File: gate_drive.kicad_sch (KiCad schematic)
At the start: 110 parts, among them J19 Conn_01x03, J20 Conn_01x03, U1 EG2131, U14 CC6920B, U2 EG2131, U20 CC6920B, U22 CC6920B, U3 CC6920B, U4 EG2131, U5 EG2131, U7 EG2131, U8 EG2131

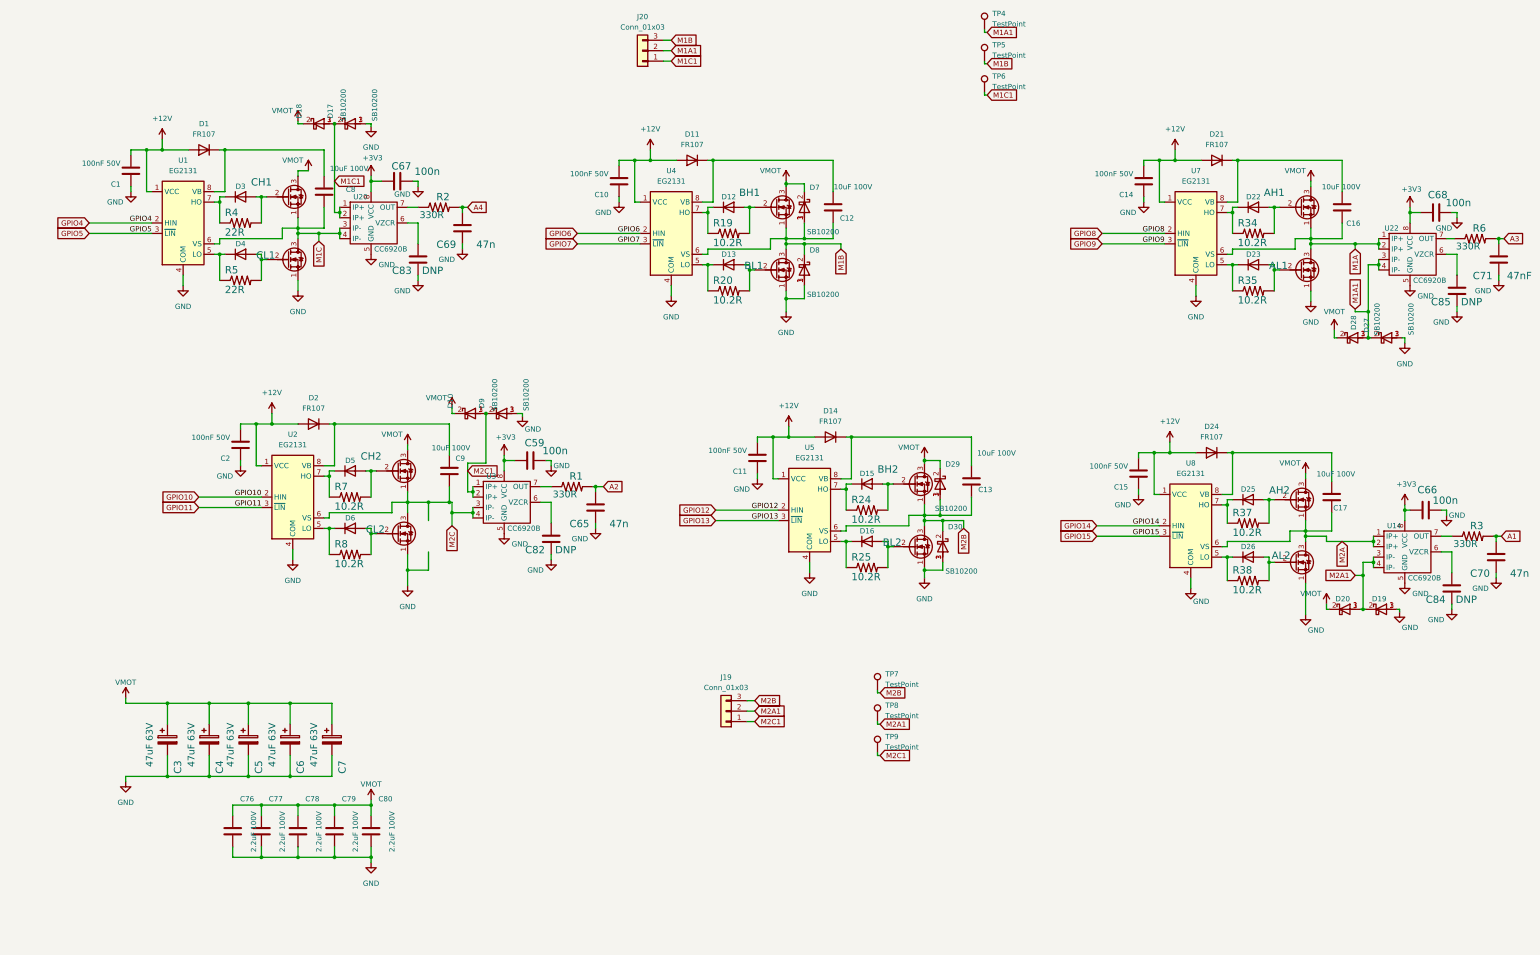
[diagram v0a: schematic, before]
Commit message: WORK IN PROGRESS updates from design review - clean schematic and PCB
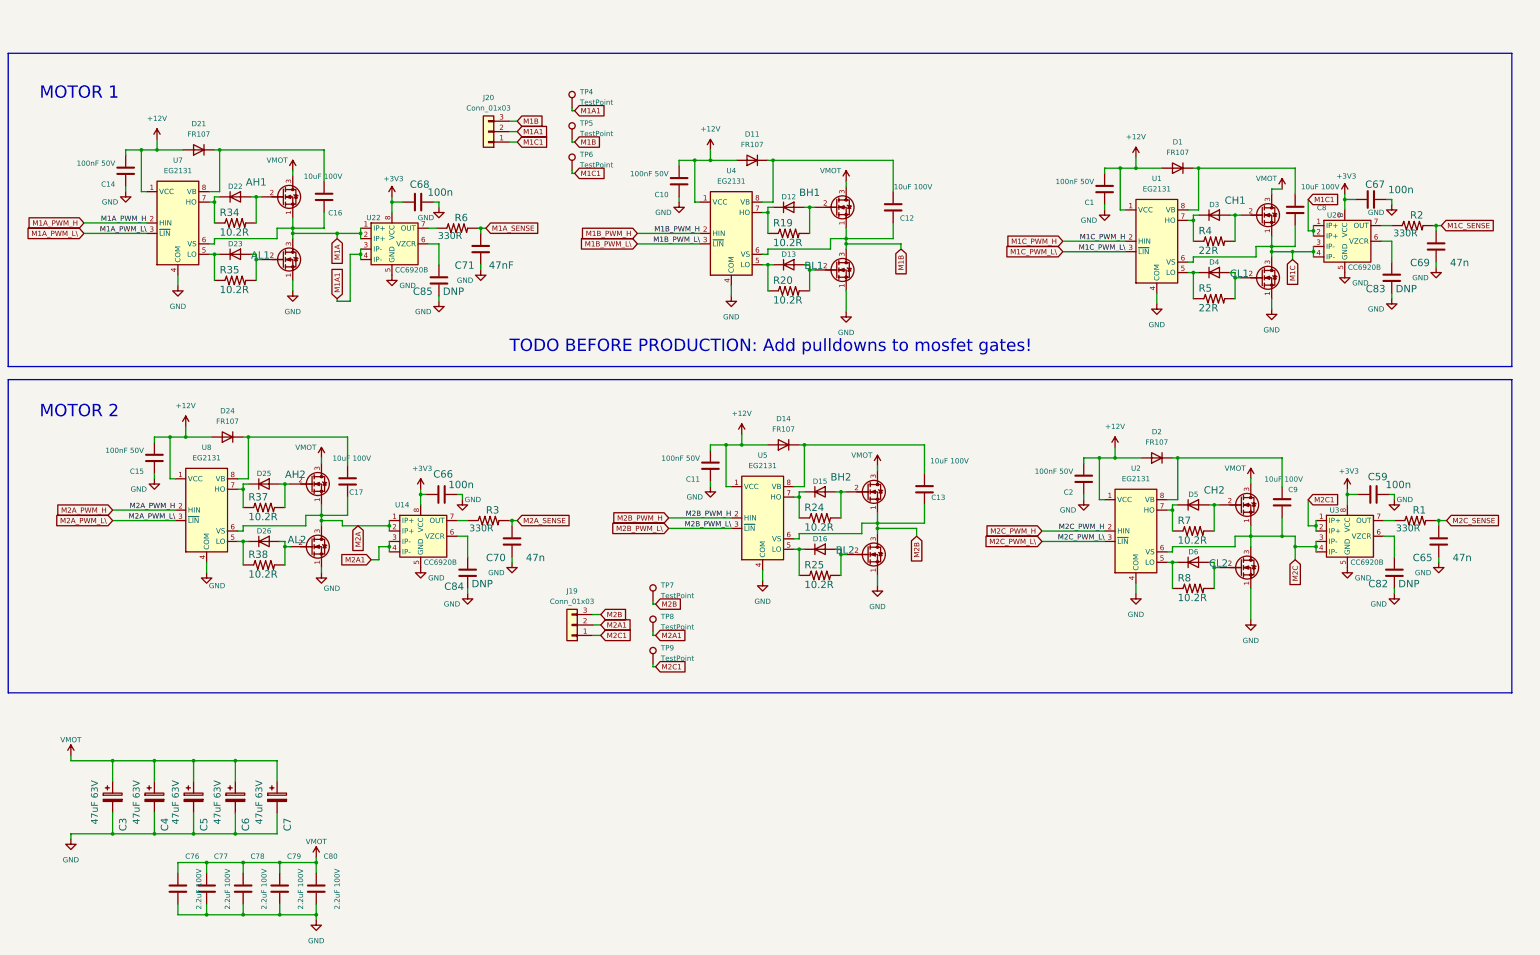
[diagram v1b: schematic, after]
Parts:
- removed D10, D17, D18, D19, D20, D27, D28, D29, D30, D7, D8, D9: SB10200, parts:TO-277_SB10200, symbol motor_parts:D_Schottky_AKA
- C12, C13, C16, C17, C8, C9: footprint Capacitor_SMD:C_2220_5650Metric -> parts:C_2220_5650Metric_expanded_paste
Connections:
- net A1 renamed M2A_SENSE
- net A2 renamed M2C_SENSE
- net A3 renamed M1A_SENSE
- net A4 renamed M1C_SENSE
- net GPIO10 renamed M2C_PWM_H
- net GPIO11 renamed M2C_PWM_L\
- net GPIO12 renamed M2B_PWM_H
- net GPIO13 renamed M2B_PWM_L\
- net GPIO14 renamed M2A_PWM_H
- net GPIO15 renamed M2A_PWM_L\
- net GPIO4 renamed M1C_PWM_H
- net GPIO5 renamed M1C_PWM_L\
- net GPIO6 renamed M1B_PWM_H
- net GPIO7 renamed M1B_PWM_L\
- net GPIO8 renamed M1A_PWM_H
- net GPIO9 renamed M1A_PWM_L\
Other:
- note added: "MOTOR 1"
- note added: "MOTOR 2"
- note added: "TODO BEFORE PRODUCTION: Add pulldowns to mosfet gates!"
- moved on the sheet: AH1, AH2, AL1, AL2, BH1, BH2, BL1, BL2, C1, C10, C11, C12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
